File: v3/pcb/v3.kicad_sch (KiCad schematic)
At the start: 425 parts, among them J1 USB_C_Receptacle_USB2.0, J2 Conn_01x21, SW1 SW_Push, SW10 SW_Push, SW100 SW_Push, SW11 SW_Push, SW12 SW_Push, SW13 SW_Push, SW14 SW_Push, SW15 SW_Push, SW16 SW_Push, SW17 SW_Push, SW18 SW_Push, SW19 SW_Push, SW2 SW_Push, SW20 SW_Push, SW21 SW_Push, SW22 SW_Push, SW23 SW_Push, SW24 SW_Push, SW25 SW_Push, SW26 SW_Push, SW27 SW_Push, SW28 SW_Push, SW29 SW_Push, SW3 SW_Push, SW30 SW_Push, SW31 SW_Push, SW32 SW_Push, SW33 SW_Push, SW34 SW_Push, SW35 SW_Push, SW36 SW_Push, SW37 SW_Push, SW38 SW_Push, SW39 SW_Push, SW4 SW_Push, SW40 SW_Push, SW41 SW_Push, SW42 SW_Push, SW43 SW_Push, SW44 SW_Push, SW45 SW_Push, SW46 SW_Push, SW47 SW_Push, SW48 SW_Push, SW49 SW_Push, SW5 SW_Push, SW50 SW_Push, SW51 SW_Push, SW52 SW_Push, SW53 SW_Push, SW54 SW_Push, SW55 SW_Push, SW56 SW_Push, SW57 SW_Push, SW58 SW_Push, SW59 SW_Push, SW6 SW_Push, SW60 SW_Push, SW61 SW_Push, SW62 SW_Push, SW63 SW_Push, SW64 SW_Push, SW65 SW_Push, SW66 SW_Push, SW67 SW_Push, SW68 SW_Push, SW69 SW_Push, SW7 SW_Push, SW70 SW_Push, SW71 SW_Push, SW72 SW_Push, SW73 SW_Push, SW74 SW_Push, SW75 SW_Push, SW76 SW_Push, SW77 SW_Push, SW78 SW_Push, SW79 SW_Push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

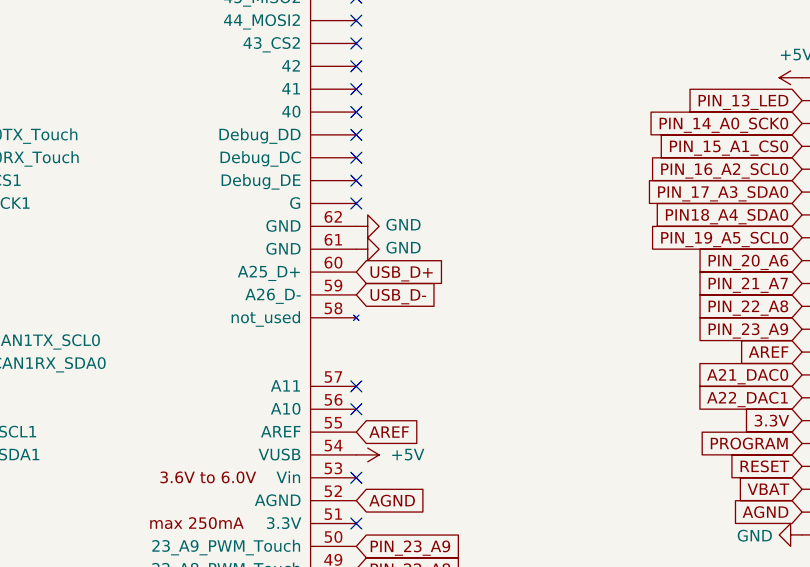
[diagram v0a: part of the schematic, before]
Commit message: Ready for production 2
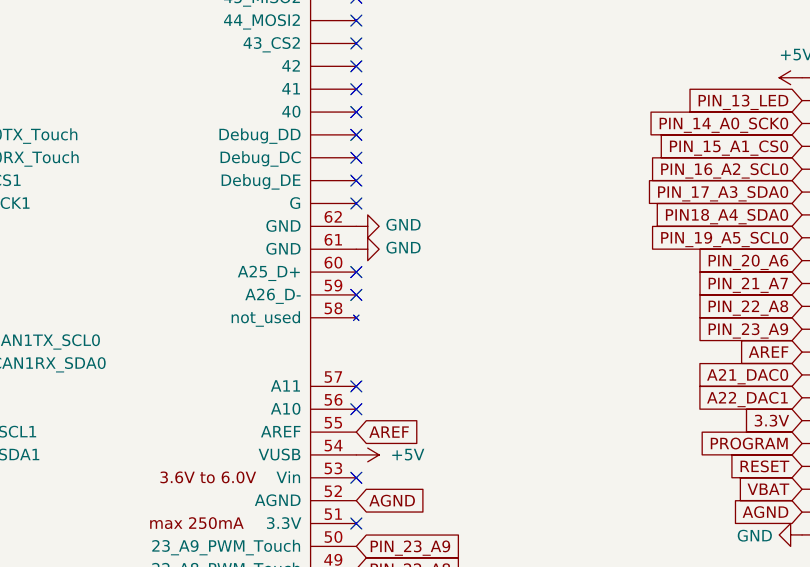
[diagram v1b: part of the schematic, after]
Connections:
- net USB_D+: no longer U1.60 (A25_D+)
- net USB_D-: no longer U1.59 (A26_D-)
- no-connect marks 36 -> 38
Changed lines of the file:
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@@
   (no_connect (at 575.31 139.7))
   (no_connect (at 575.31 68.58))
+  (no_connect (at 575.31 127))
   (no_connect (at 684.53 66.04))
   (no_connect (at 575.31 60.96))
@@
   (no_connect (at 516.89 157.48))
   (no_connect (at 575.31 149.86))
+  (no_connect (at 575.31 129.54))
   (no_connect (at 575.31 93.98))
   (wire (pts (xy 325.12 297.18) (xy 340.36 297.18))
@@
     )
   )
-  (global_label "USB_D+" (shape input) (at 575.31 127 0) (fields_autoplaced)
-    (effects (font (size 1.27 1.27)) (justify left))
-    (property "Intersheet References" "${INTERSHEET_REFS}" (id 0) (at 585.3431 126.9206 0)
-      (effects (font (size 1.27 1.27)) (justify left) hide)
-    )
-  )
   (global_label "COL16" (shape input) (at 322.58 53.34 90) (fields_autoplaced)
     (effects (font (size 1.27 1.27)) (justify left))
@@
     )
   )
-  (global_label "USB_D-" (shape input) (at 575.31 129.54 0) (fields_autoplaced)
-    (effects (font (size 1.27 1.27)) (justify left))
-    (property "Intersheet References" "${INTERSHEET_REFS}" (id 0) (at 585.3431 129.4606 0)
-      (effects (font (size 1.27 1.27)) (justify left) hide)
-    )
-  )
